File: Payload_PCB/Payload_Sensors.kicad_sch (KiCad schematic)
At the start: 8 parts

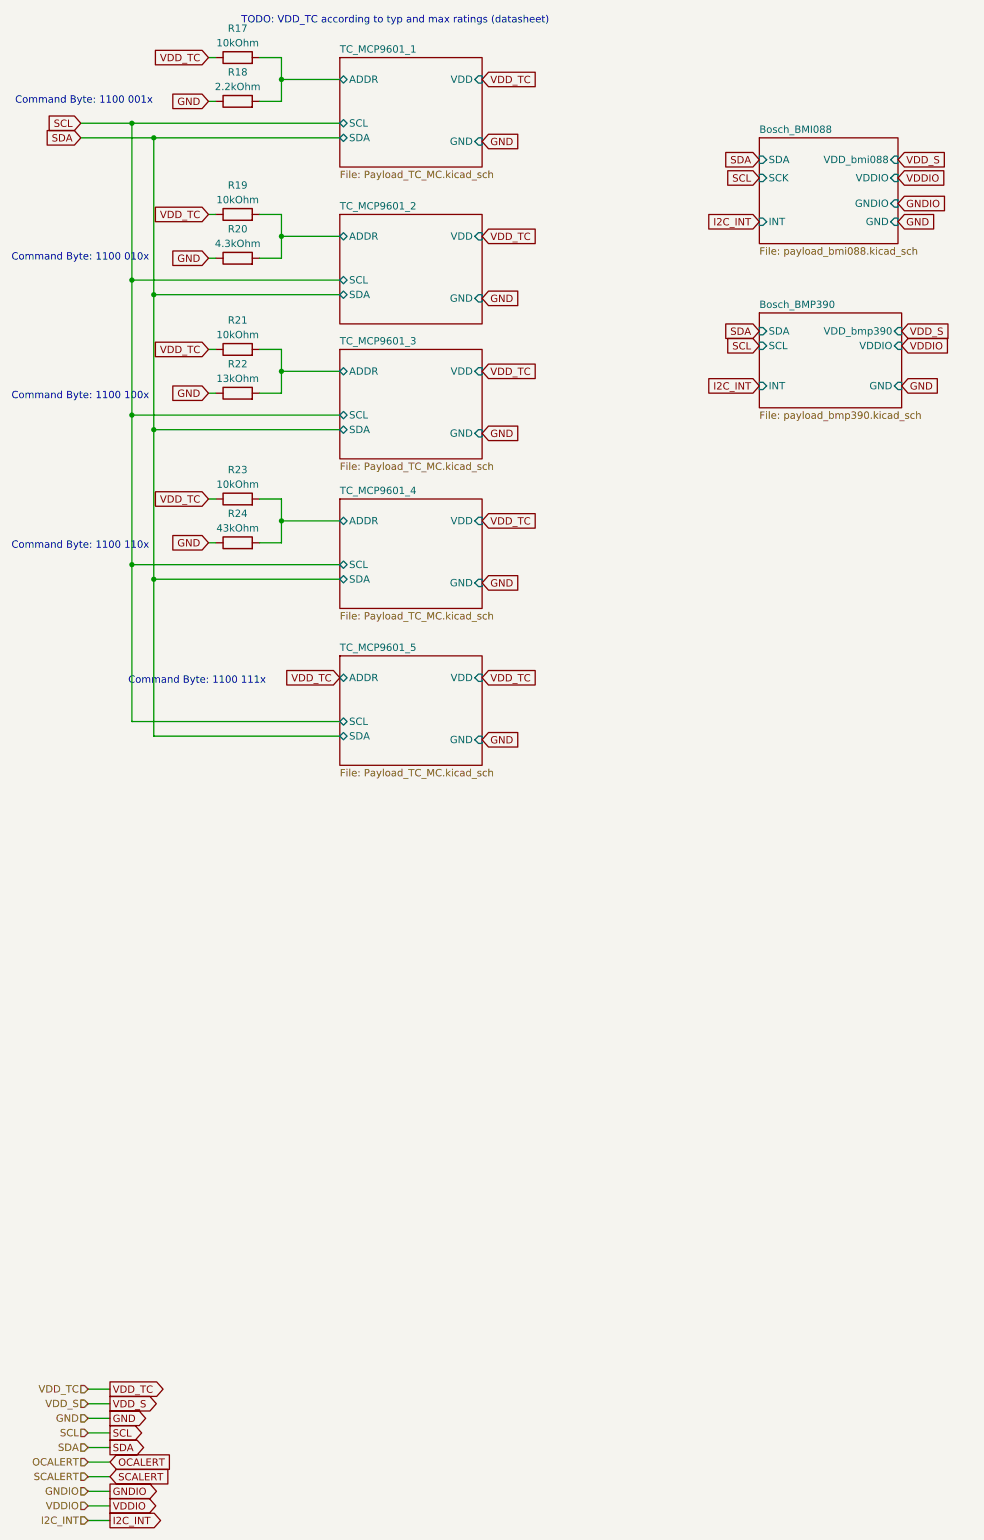
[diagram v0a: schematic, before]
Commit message: Added some actual parts
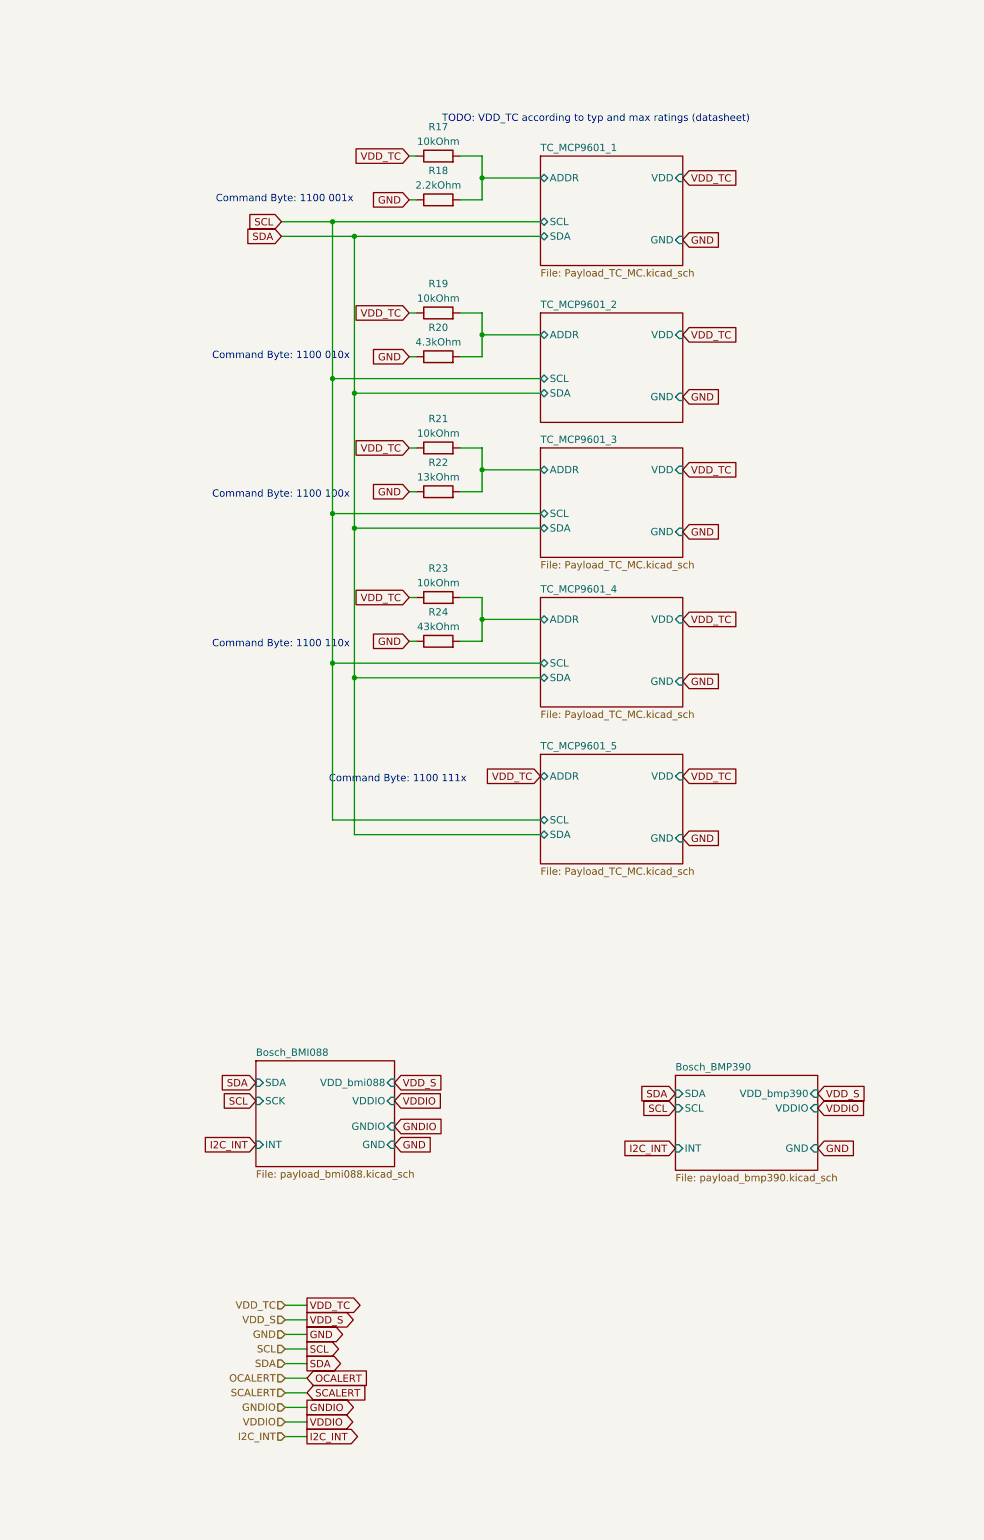
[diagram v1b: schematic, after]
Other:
- title: (none) -> Sensor Modules
- moved on the sheet: R17, R18, R19, R20, R21, R22, R23, R24
